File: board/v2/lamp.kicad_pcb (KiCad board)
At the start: 4 copper layers, 28 x 28 mm, 43 parts, among them J1 Conn_01x01_Female, J2 Conn_01x01_Female, J3 Conn_01x01_Female, J4 Conn_01x01_Female, J5 Conn_01x01_Female, J6 Conn_01x01_Female, J7 Conn_01x01_Female, J8 Conn_ARM_JTAG_SWD_10, Q1 SiA453EDJ, U1 STM32G071GxU, U2 TLV333, U3 LP2985-33, U4 LMR23625

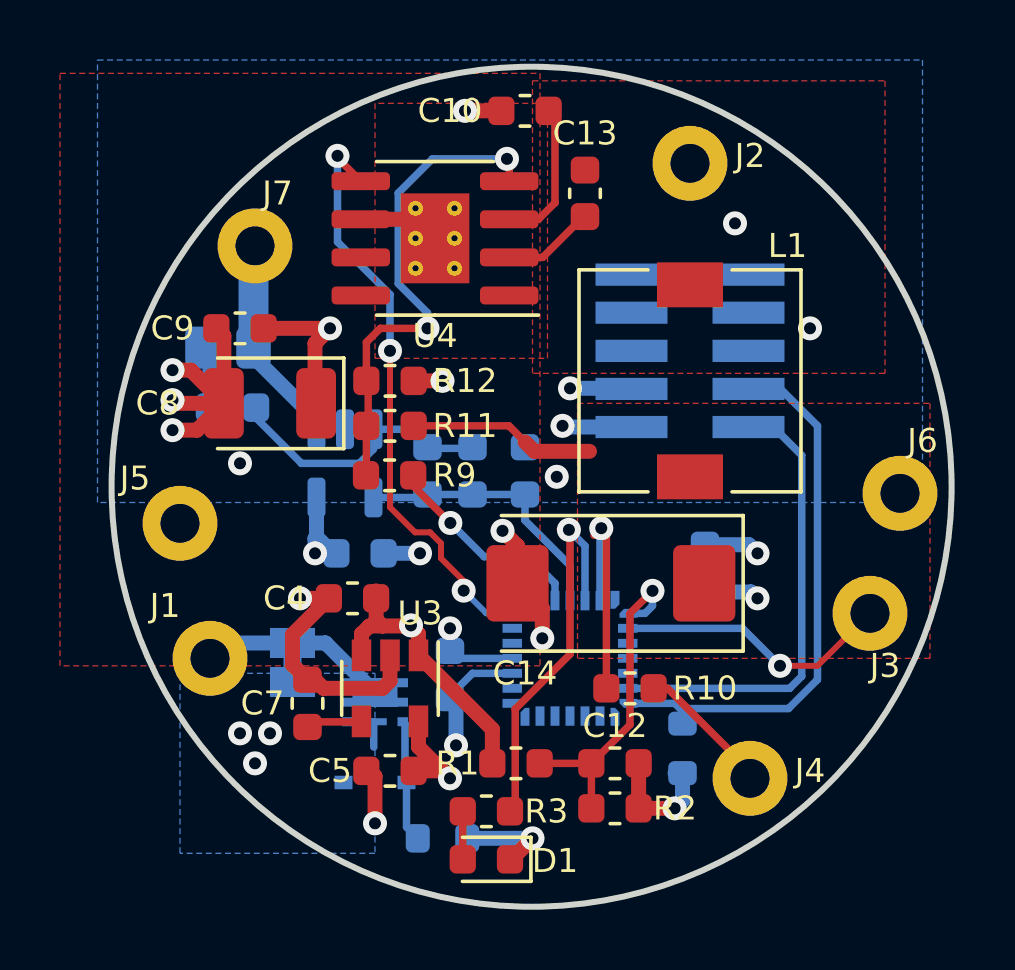
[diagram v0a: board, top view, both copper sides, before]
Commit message: hardware: More fiddling
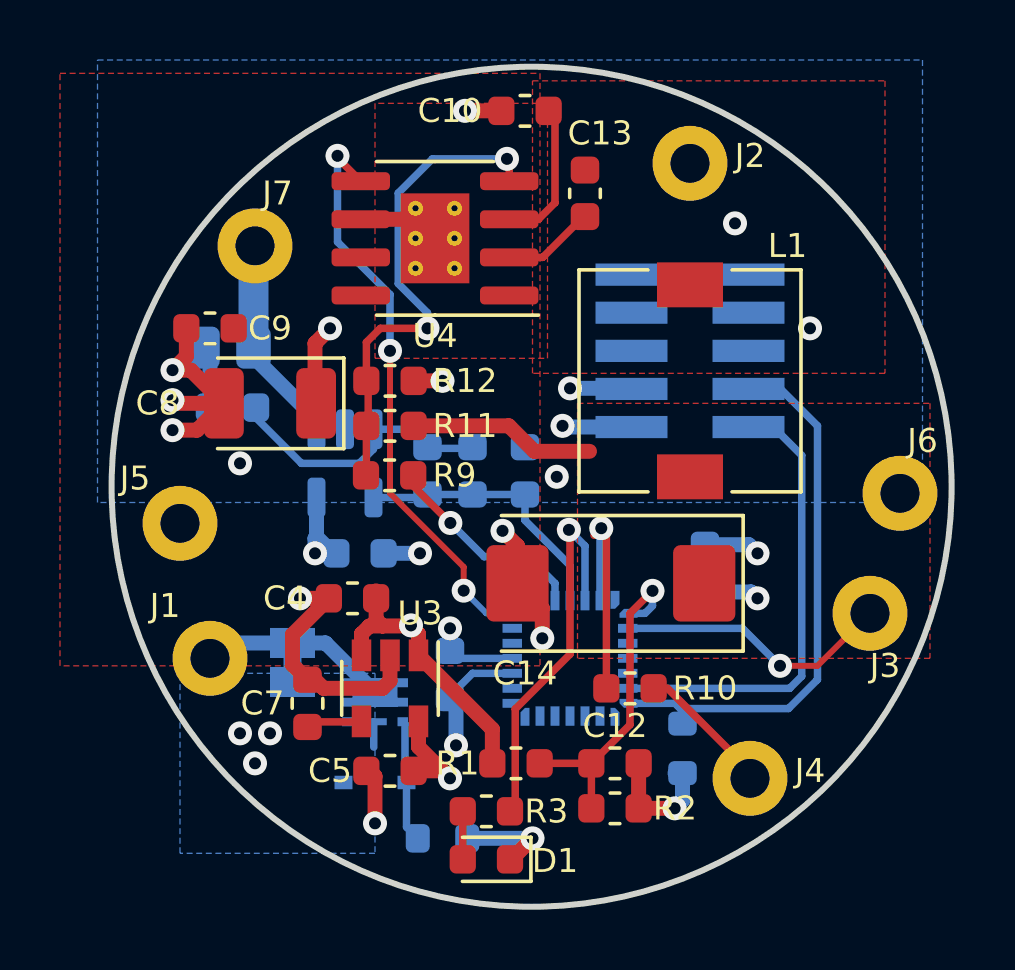
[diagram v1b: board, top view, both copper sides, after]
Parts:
- moved C9 1.00 mm to (125.0, 78.5)
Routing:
- net /Vin: track 15.4 -> 13.0 mm
- net GND: track 44.1 -> 43.0 mm
- net /Vbat: track 6.40 -> 5.67 mm
